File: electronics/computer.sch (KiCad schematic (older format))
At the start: 3 parts, among them U38 74LS04

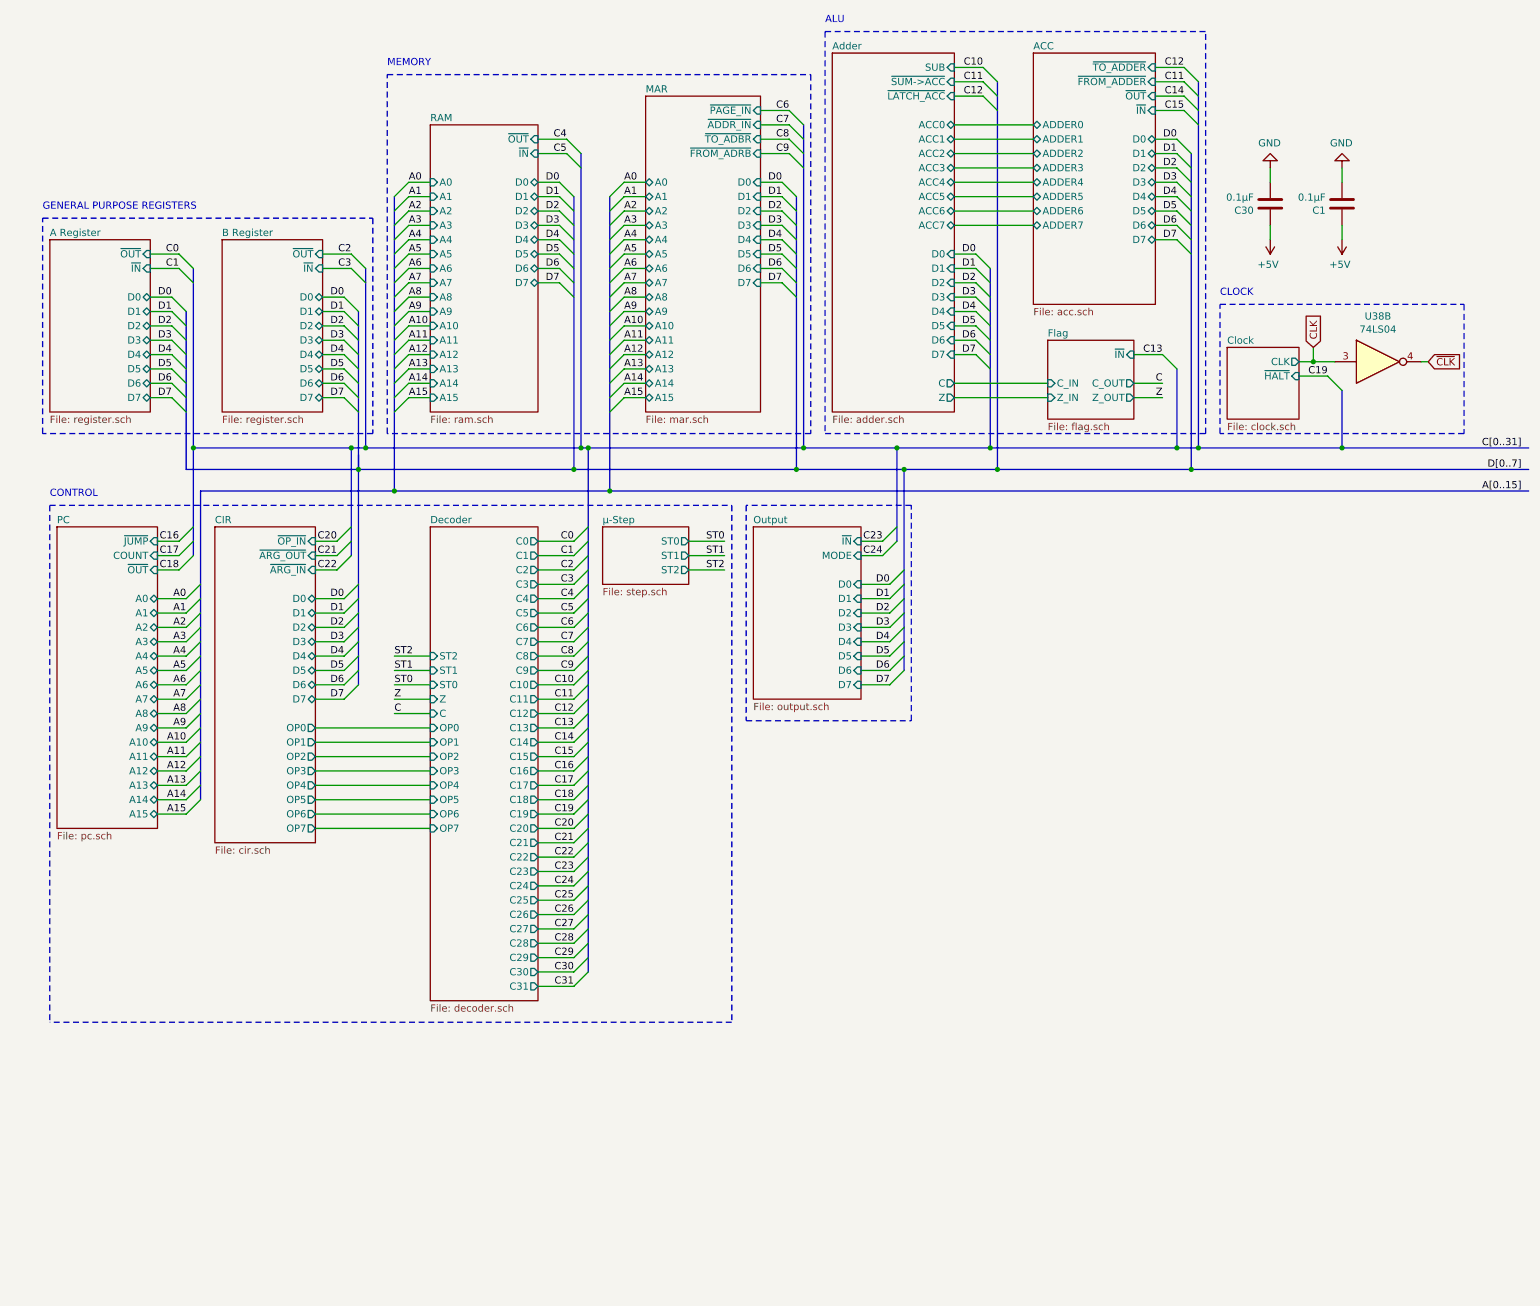
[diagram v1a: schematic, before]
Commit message: Some initial electronics design
Not everything done yet, just committing to show progress and to get the changes out of the way.
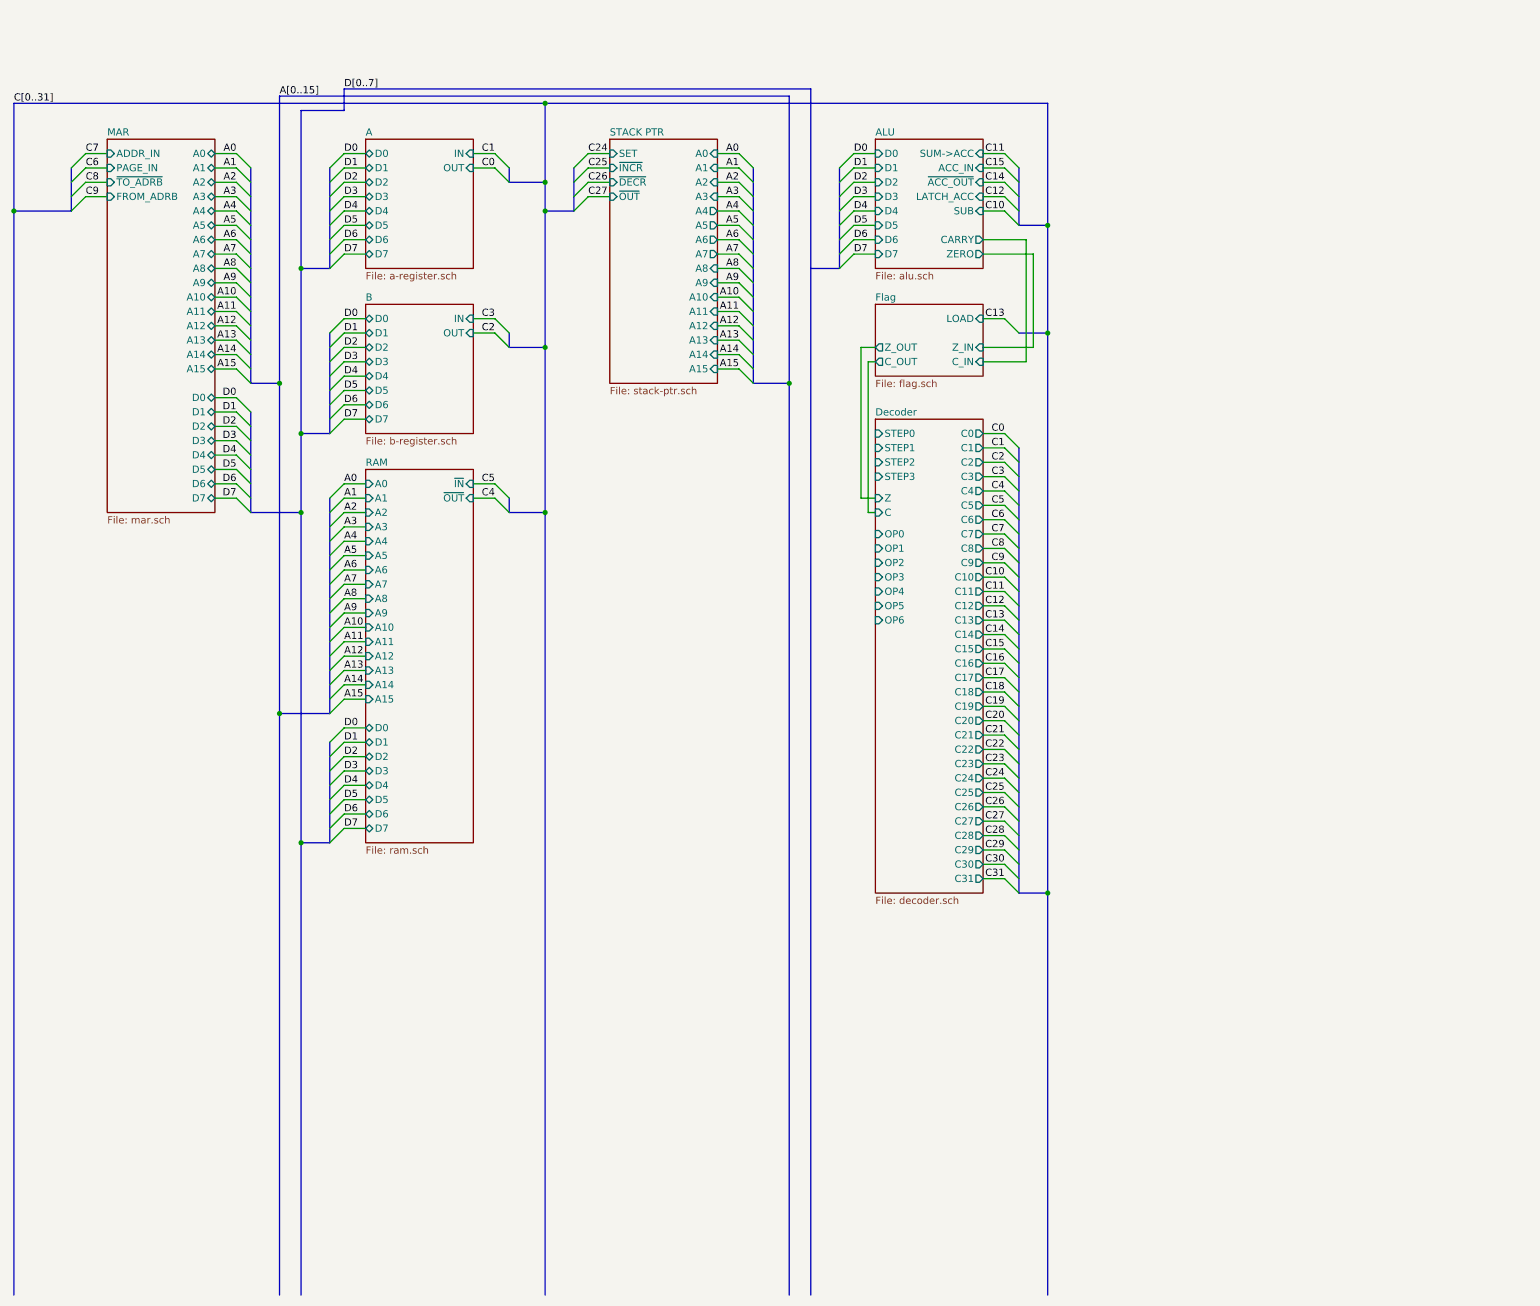
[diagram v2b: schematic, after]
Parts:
- removed C1, C30: 0.1µF, Capacitor_THT:CP_Radial_D4.0mm_P1.50mm, symbol Device:C
- removed U38: 74LS04, Package_DIP:DIP-14_W7.62mm, symbol 74xx:74LS04
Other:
- note removed: "ALU"
- note removed: "CLOCK"
- note removed: "CONTROL"
- note removed: "GENERAL PURPOSE REGISTERS"
- note removed: "MEMORY"
